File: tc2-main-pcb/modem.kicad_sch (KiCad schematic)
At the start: 12 parts, among them J11 Conn_01x08, J7 Screw_Terminal_01x01, U12 SIM7600G-H-M.2

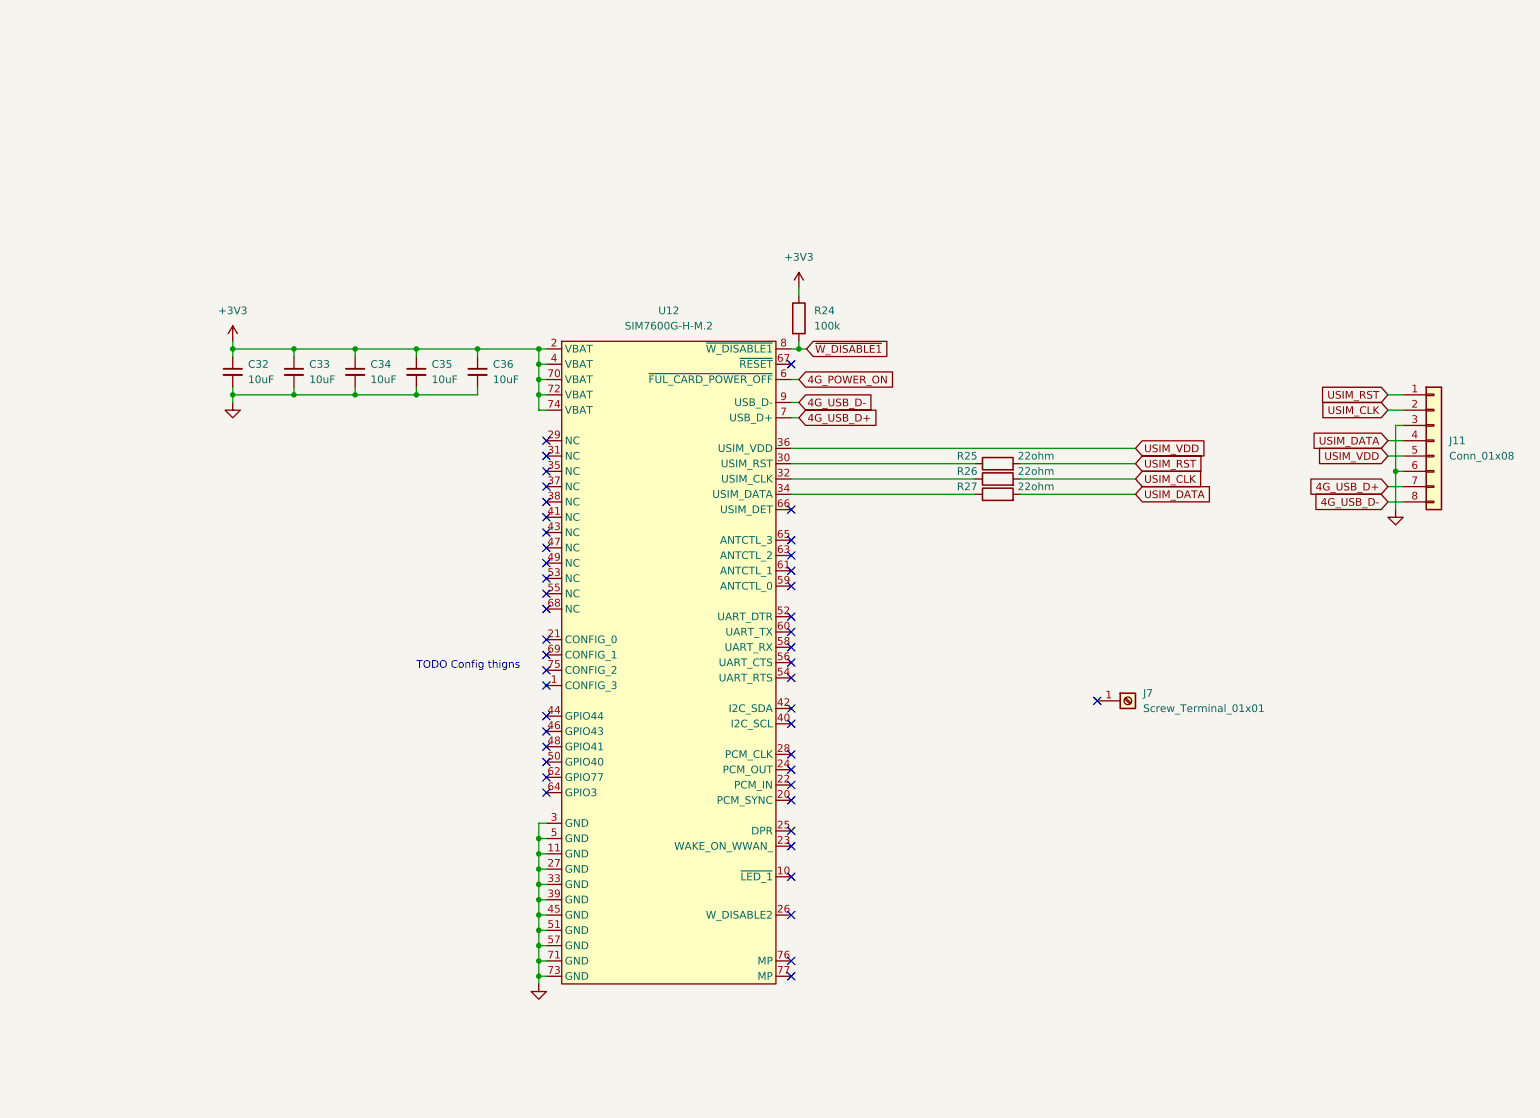
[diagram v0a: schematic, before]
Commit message: P3-Nov release
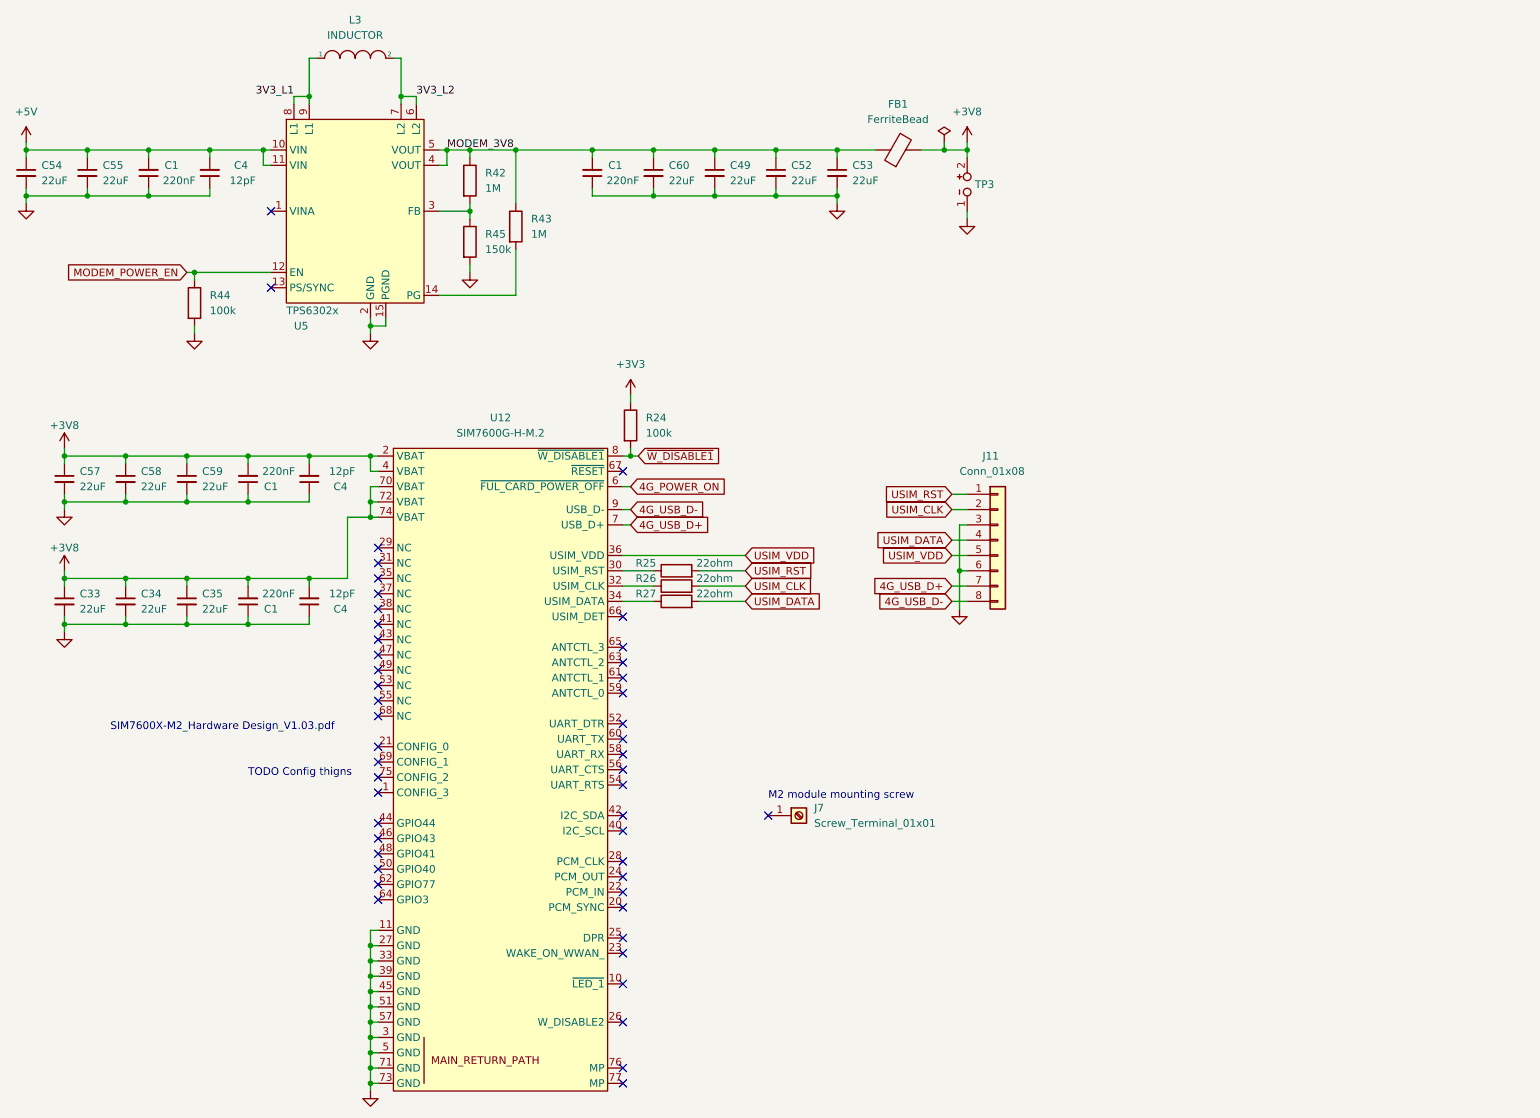
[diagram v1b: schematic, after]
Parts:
- removed C32, C36: 10uF, Capacitor_SMD:C_0603_1608Metric, symbol Device:C_Small
- added C1 (x4): 220nF, Capacitor_SMD:C_0402_1005Metric, symbol Device:C_Small
- added C4 (x3): 12pF, Capacitor_SMD:C_0402_1005Metric, symbol Device:C_Small
- added C49, C52, C53, C54, C55, C57, C58, C59, C60: 22uF, Capacitor_SMD:C_0603_1608Metric, symbol Device:C_Small
- added FB1: FerriteBead, Inductor_SMD:L_0805_2012Metric, symbol Device:FerriteBead
- added L3: INDUCTOR, Inductor_SMD:L_1008_2520Metric, symbol cacophony-library:Power_Inductor
- added R42, R43: 1M, Resistor_SMD:R_0402_1005Metric, symbol Device:R
- added R44: 100k, Resistor_SMD:R_0402_1005Metric, symbol Device:R
- added R45: 150k, Resistor_SMD:R_0402_1005Metric, symbol Device:R
- added TP3: TP_2P, cacophony-library:test-point-2p, symbol cacophony-library:TestPoint_2Pole
- added U5: TPS6302x, cacophony-library:VSON-14_L4.0-W3.0-P0.50-BL-EP_TI_DSJ, symbol cacophony-library:TPS6302x
- C33, C34, C35: value 10uF -> 22uF; LCSC C19702 -> C2980159
- J7: footprint cacophony-library:SMD_BD4.4-L4.4-D2.8 -> cacophony-library:M2_modem_mount_screw; LCSC C2928178 -> C2928176
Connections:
- net +3V3: no longer C33.1, C34.1, C35.1, U12.2 (VBAT), U12.4 (VBAT), U12.70 (VBAT), U12.72 (VBAT), U12.74 (VBAT)
- net GND: now also C1.1, C1.1, C1.1, C1.1, C4.1, C4.1, C4.1, C49.2, C52.2, C53.2, C54.2, C55.2, C57.2, C58.2, C59.2, C60.2, R44.2, R45.2, TP3.1, U5.15 (PGND), U5.2 (GND)
- new net: R43.2, U5.14 (PG)
- new net: R42.2, R45.1, U5.3 (FB)
- new net +3V8: C1.2, C1.2, C33.1, C34.1, C35.1, C4.2, C4.2, C57.1, C58.1, C59.1, FB1.2, TP3.2, U12.2 (VBAT), U12.4 (VBAT), U12.70 (VBAT), U12.72 (VBAT), U12.74 (VBAT)
- new net +5V: C1.2, C4.2, C54.1, C55.1, U5.10 (VIN), U5.11 (VIN)
- new net 3V3_L1: L3.1, U5.8 (L1), U5.9 (L1)
- new net 3V3_L2: L3.2, U5.6 (L2), U5.7 (L2)
- new net MODEM_3V8: C1.2, C49.1, C52.1, C53.1, C60.1, FB1.1, R42.1, R43.1, U5.4 (VOUT), U5.5 (VOUT)
- new net MODEM_POWER_EN: R44.1, U5.12 (EN)
- no-connect marks 46 -> 48
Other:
- note added: "M2 module mounting screw"
- note added: "SIM7600X-M2_Hardware Design_V1.03.pdf"
- moved on the sheet: J11, J7, R24, R25, R26, R27
